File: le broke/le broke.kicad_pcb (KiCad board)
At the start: 2 copper layers, 100 x 83 mm, 43 parts, among them SW1 SW_Push, U1 ProMicro

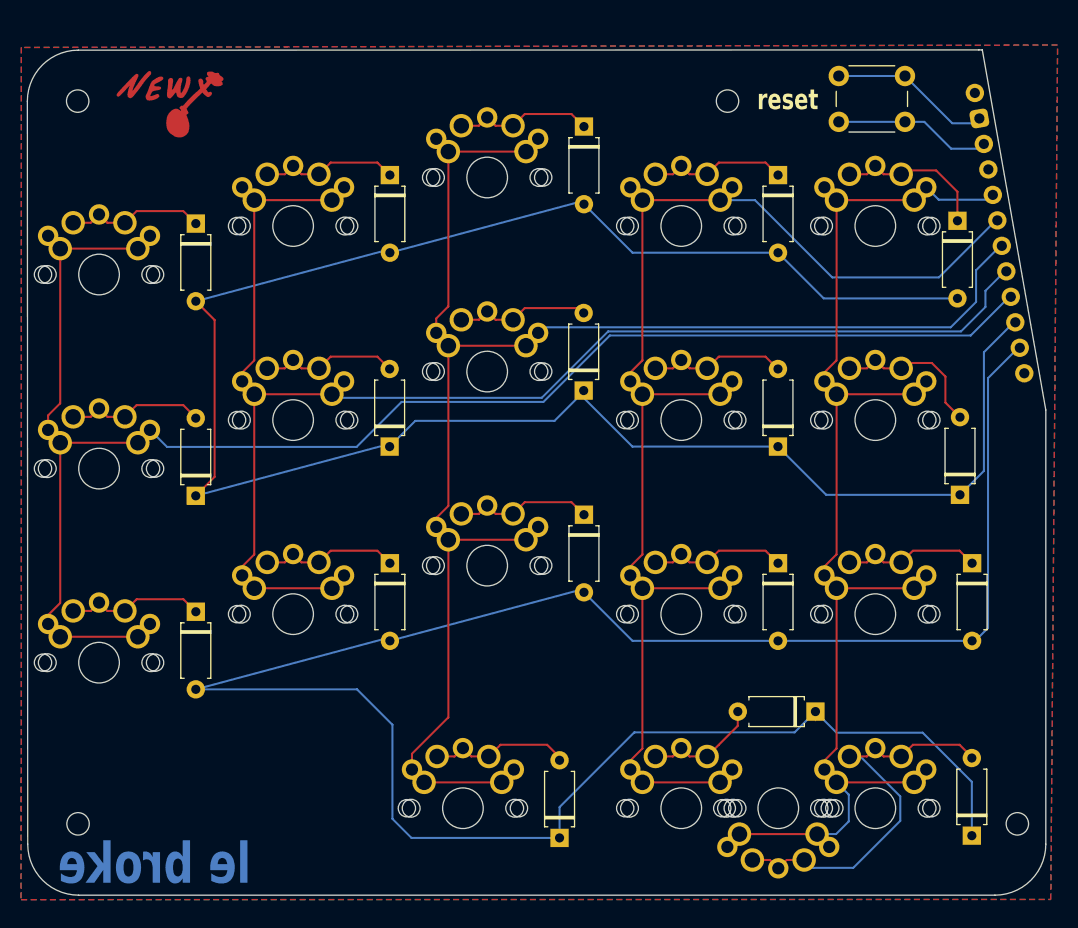
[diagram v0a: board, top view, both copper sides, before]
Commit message: new pcb etc
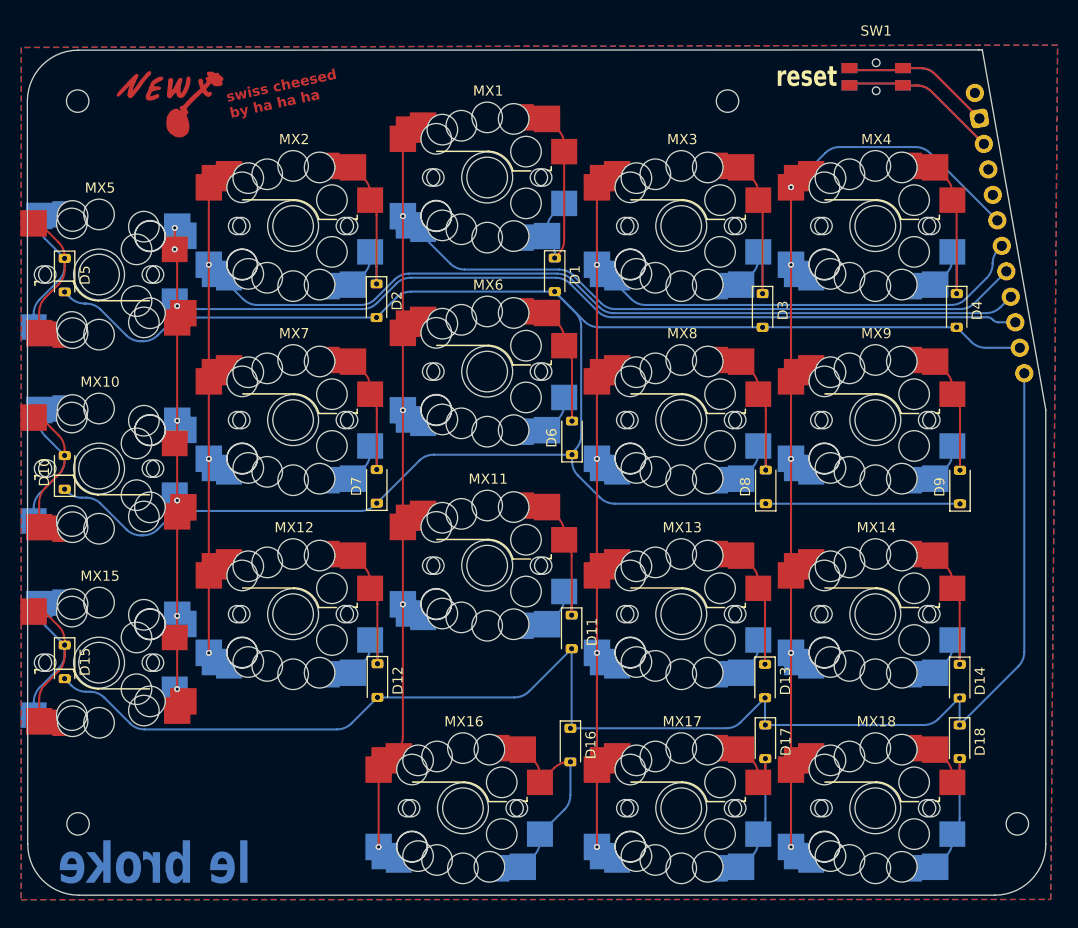
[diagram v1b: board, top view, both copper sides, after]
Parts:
- removed the MX18 at (166.9, 125.5)
- D1, D10, D11, D12, D13, D14, D15, D16, D17, D18, D2, D3, D4, D5, D6, D7, D8, D9: footprint isaacscollection:D_A-405_P7.62mm_Horizontal -> zackforbing:D_SOD-123
- MX1, MX11, MX12, MX13, MX14, MX16, MX17, MX18, MX2, MX3, MX4, MX6, MX7, MX8, MX9: footprint marbastlib-mx:SW_MX_1u_rev -> fingerpunch:gateron-ks27-choc-v1-mx-hotswap-reversible
- MX10, MX15, MX5: footprint marbastlib-mx:SW_MX_1u_rev -> fingerpunch:gateron-ks27-choc-v1-mx-hotswap-reversible edge preferred
- SW1: footprint Button_Switch_THT:SW_PUSH_6mm -> zackforbing:Panasonic_EVQPUL_EVQPUC PTH
- moved D1 14.8 mm to (144.9, 73.1)
- moved D5 13.8 mm to (96.8, 73.1)
- moved D15 13.8 mm to (96.8, 111.1)
- moved D3 13.4 mm to (165.3, 76.6)
- moved D10 13.1 mm to (96.8, 92.5)
- moved D2 12.4 mm to (127.4, 75.6)
- moved D14 11.6 mm to (184.7, 113.0)
- moved D13 11.6 mm to (165.6, 113.0)
- moved D12 11.6 mm to (127.5, 112.9)
- moved D11 11.6 mm to (146.6, 108.2)
- moved D18 9.29 mm to (184.7, 118.9), turned to -90 degrees
- moved D16 9.18 mm to (146.5, 119.3), turned to -90 degrees
- moved D4 8.80 mm to (184.4, 76.6)
- moved D17 5.74 mm to (165.6, 118.9), turned to -90 degrees
- moved D6 4.78 mm to (146.6, 89.1)
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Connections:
- net Net-(SW1-Pad1) renamed GND
- net Net-(U1-RST) renamed RST
- U1 pad 17: COL4 -> unconnected-(U1-F4-Pad17)
- U1 pad 18: COL3 -> COL4
- U1 pad 19: COL2 -> COL3
- U1 pad 20: COL1 -> COL2
- U1 pad 21: COL0 -> COL1
- U1 pad 22: ROW0 -> COL0
- U1 pad 23: ROW1 -> ROW0
- U1 pad 24: unconnected-(U1-B6-Pad24) -> ROW1
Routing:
- net ROW1: track 214.1 -> 145.2 mm
- net Net-(D18-A): track 40.1 -> 17.8 mm
- net COL4: track 108.3 -> 89.8 mm, vias 0 -> 5
- net COL0: track 150.7 -> 133.5 mm, vias 0 -> 7
- net RST: track 15.7 -> 31.3 mm
- net GND: track 16.0 -> 29.7 mm
- net Net-(D15-K): track 13.7 -> 26.5 mm
- net Net-(D10-A): track 13.7 -> 26.1 mm
- net Net-(D5-K): track 13.7 -> 26.0 mm
- net COL2: track 143.7 -> 134.6 mm, vias 0 -> 4
- net COL3: track 118.0 -> 109.1 mm, vias 0 -> 4
- net ROW0: track 202.8 -> 211.6 mm
- net Net-(D3-K): track 13.7 -> 21.3 mm
- net Net-(D4-K): track 15.2 -> 22.6 mm
- net Net-(D1-K): track 13.7 -> 20.7 mm
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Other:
- board text added: "swiss cheesed by ha ha ha"
